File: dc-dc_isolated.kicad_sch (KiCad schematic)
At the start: 11 parts, among them U801 CMP6793RE

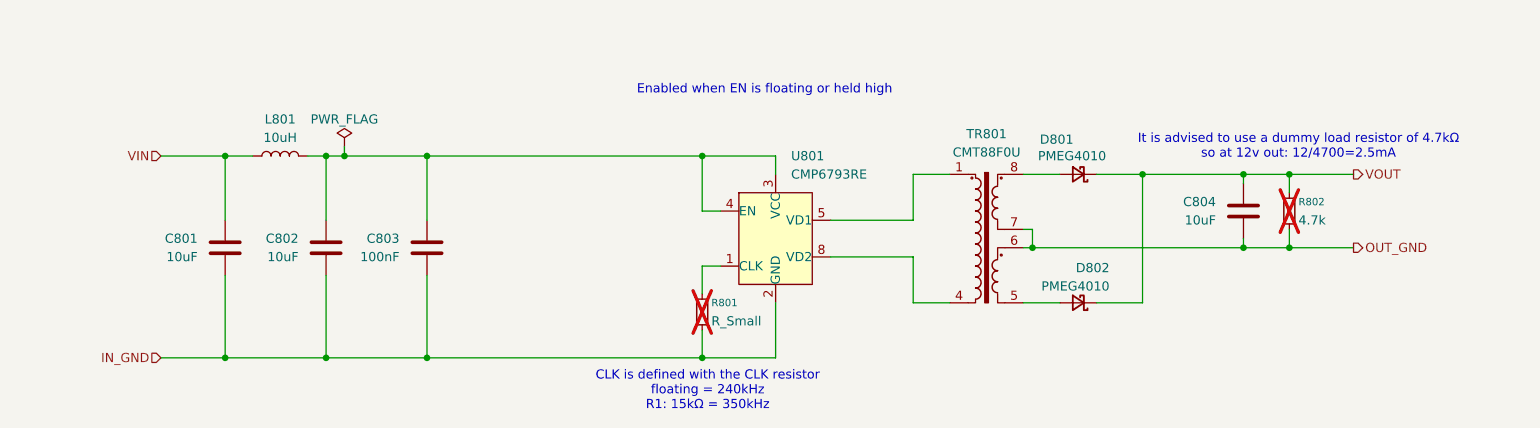
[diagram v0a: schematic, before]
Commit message: First layout complete - DRC not clear yet.
Signed-off-by: Jean Alinei <jean.alinei@owntech.org>
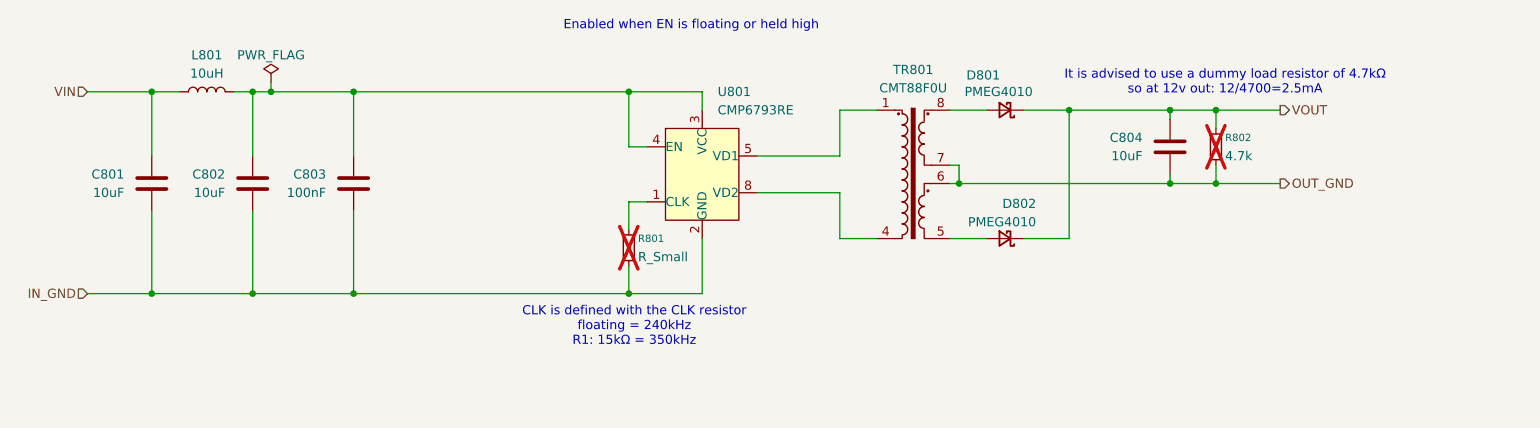
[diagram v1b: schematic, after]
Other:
- moved on the sheet: C801, C802, C803, C804, D801, D802, L801, R801, R802, TR801, U801

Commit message: Found IC for ORing function. Added all LCSC refs. Found proper header stackup.
Signed-off-by: Jean Alinei <jean.alinei@owntech.org>
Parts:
- TR801: LCSC (none) -> C37648313
